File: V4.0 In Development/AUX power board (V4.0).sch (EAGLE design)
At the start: 95 parts, among them U1 ATMEGA328P_TQFP, U2 TPS5405DR

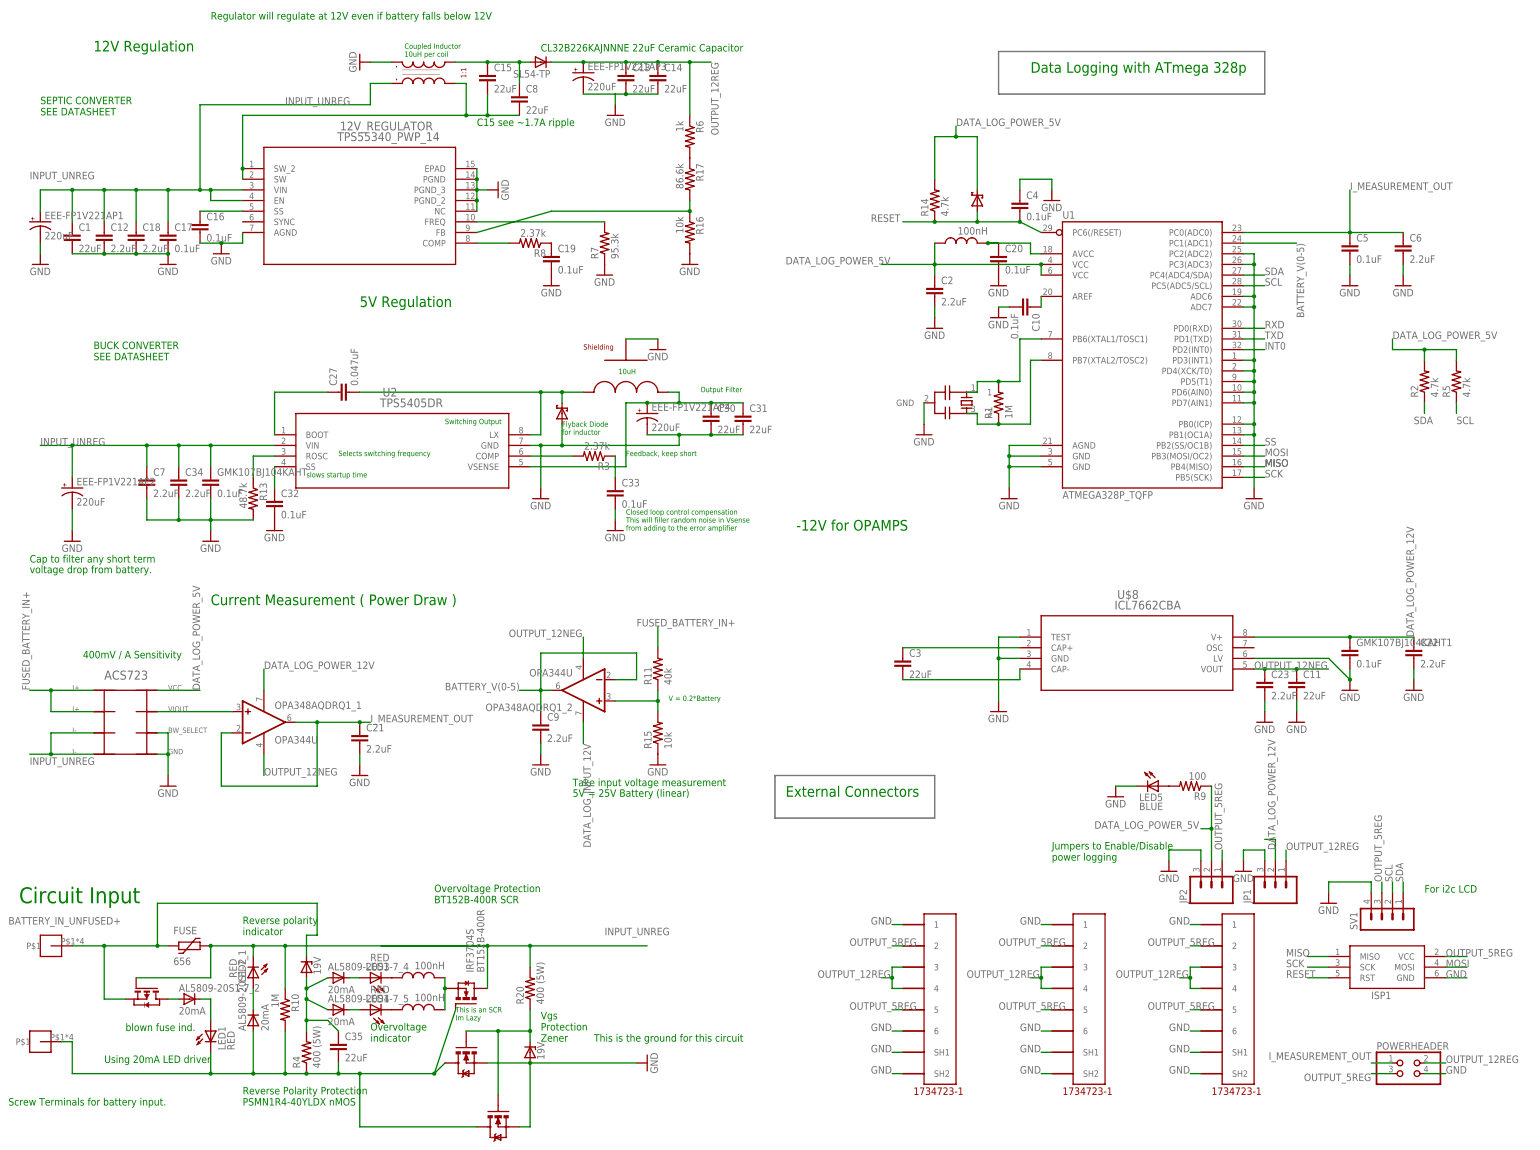
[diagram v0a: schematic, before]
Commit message: Trying this commit again
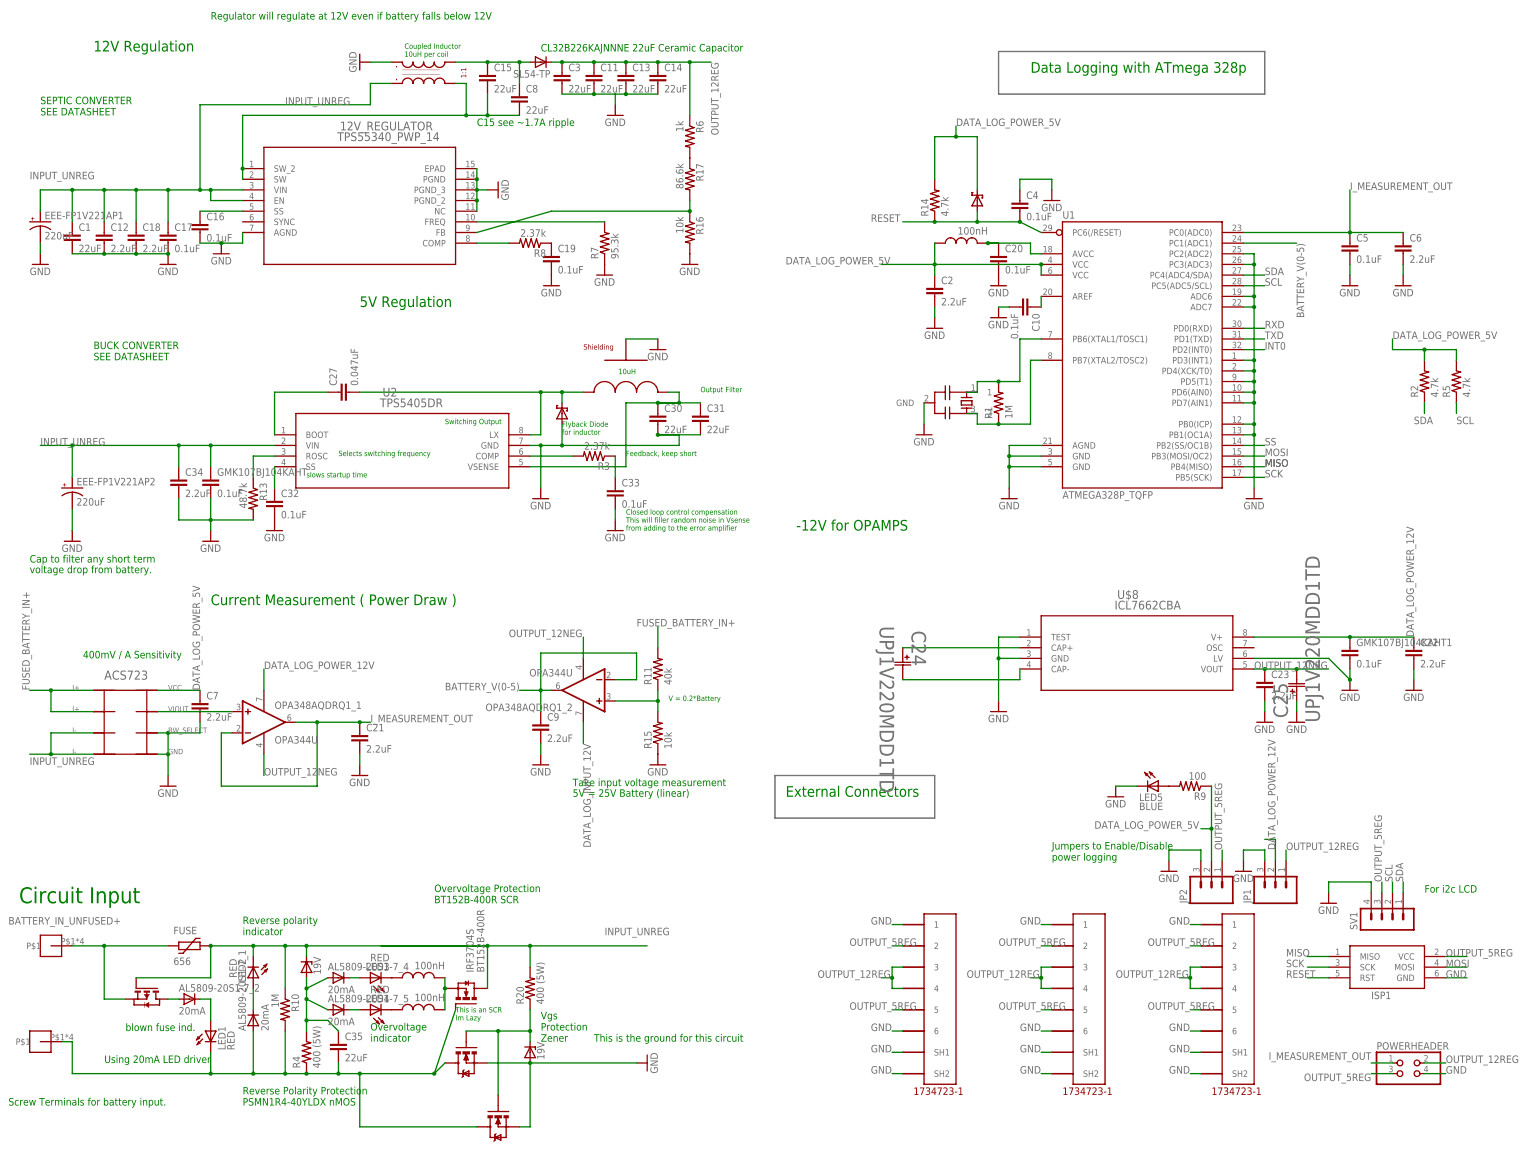
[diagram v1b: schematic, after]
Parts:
- removed EEE-FP1V221AP3, EEE-FP1V221AP4: 220uF, rcl:CPOL-US175TMP-0808
- added C24, C25: UPJ1V220MDD1TD, UPJ1V220MDD1TD:UPJ1V220MDD1TD
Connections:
- net BATTERY_IN_UNFUSED+: no longer 1N5354BRLG.C
- net DATA_LOG_POWER_5V: now also C7.1
- net GND: now also C25.11, C3.2; no longer EEE-FP1V221AP3.-, EEE-FP1V221AP4.-
- net INPUT_UNREG: now also 1N5354BRLG.C; no longer C7.1
- net N$11: now also C24.22; no longer C3.2
- net N$16: now also C24.11; no longer C3.1
- net N$26: no longer EEE-FP1V221AP4.+
- net OUTPUT_12NEG: now also C25.22; no longer C11.1
- net OUTPUT_12REG: now also C11.1, C3.1; no longer EEE-FP1V221AP3.+
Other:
- moved on the sheet: C11, C3, C30, C31, C7

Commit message: when git fails to sync
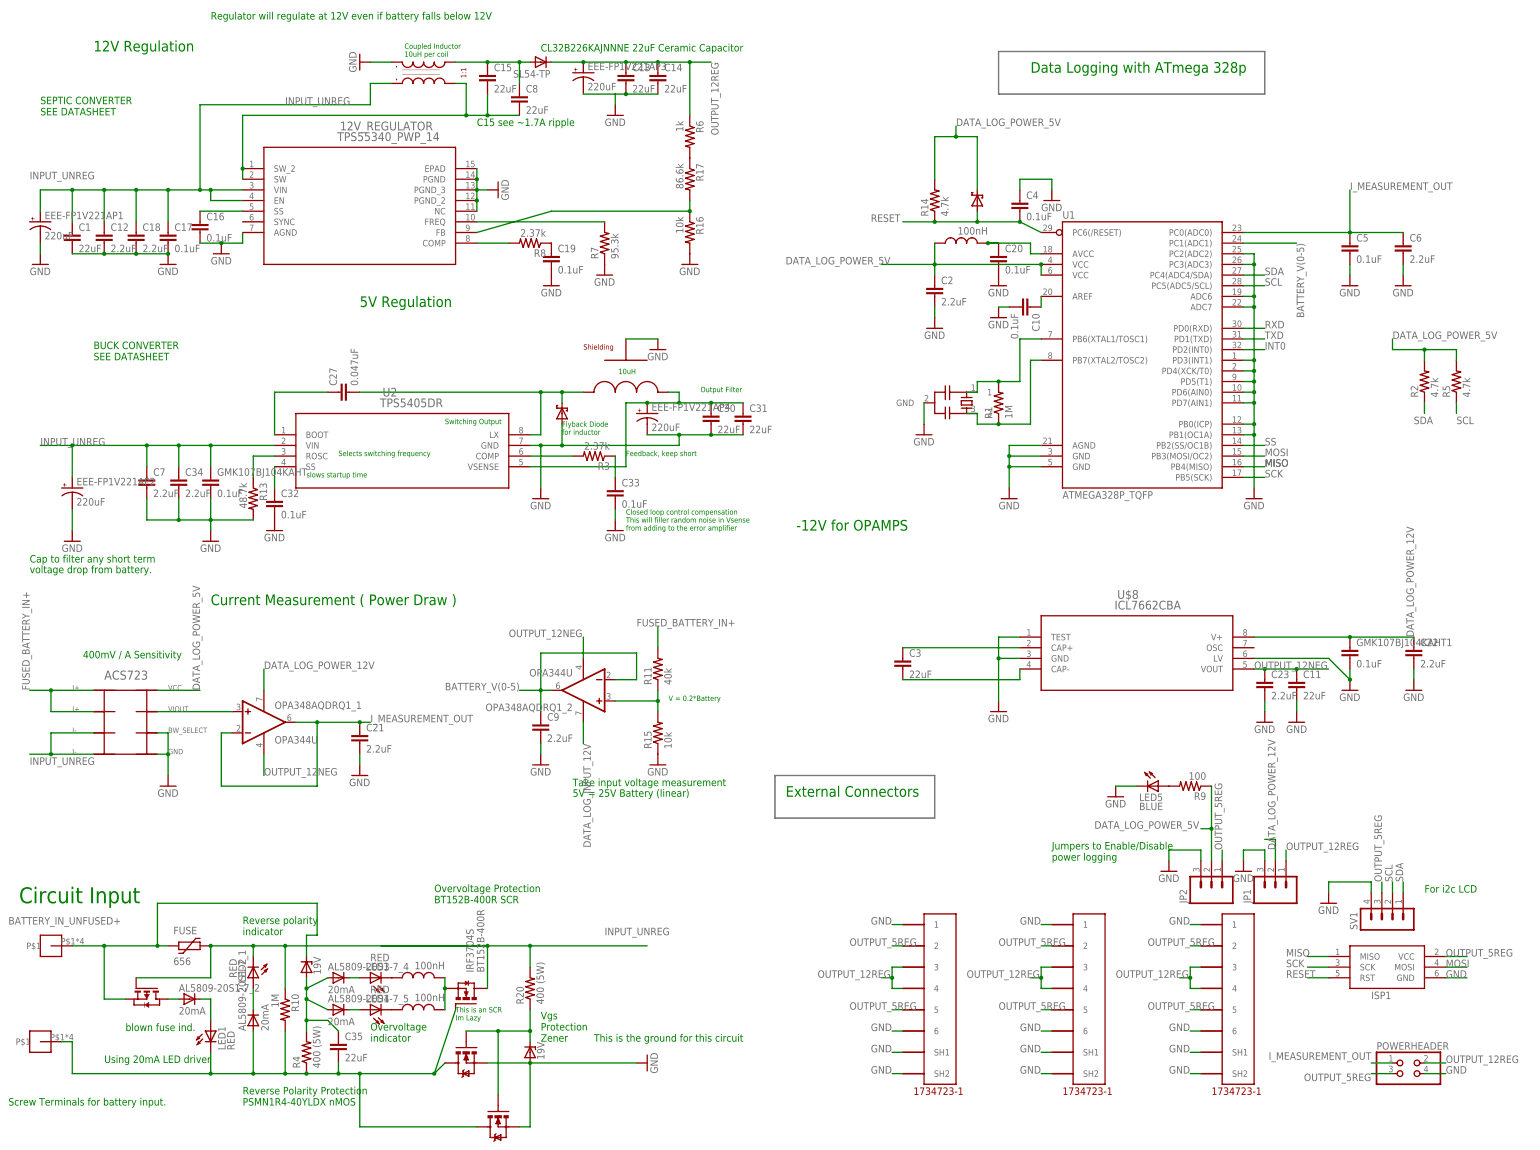
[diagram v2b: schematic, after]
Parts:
- removed C24, C25: UPJ1V220MDD1TD, UPJ1V220MDD1TD:UPJ1V220MDD1TD
- added EEE-FP1V221AP3, EEE-FP1V221AP4: 220uF, rcl:CPOL-US175TMP-0808
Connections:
- net BATTERY_IN_UNFUSED+: now also 1N5354BRLG.C
- net DATA_LOG_POWER_5V: no longer C7.1
- net GND: now also EEE-FP1V221AP3.-, EEE-FP1V221AP4.-; no longer C25.11, C3.2
- net INPUT_UNREG: now also C7.1; no longer 1N5354BRLG.C
- net N$11: now also C3.2; no longer C24.22
- net N$16: now also C3.1; no longer C24.11
- net N$26: now also EEE-FP1V221AP4.+
- net OUTPUT_12NEG: now also C11.1; no longer C25.22
- net OUTPUT_12REG: now also EEE-FP1V221AP3.+; no longer C11.1, C3.1
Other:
- moved on the sheet: C11, C3, C30, C31, C7
